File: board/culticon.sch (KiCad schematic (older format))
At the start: 32 parts

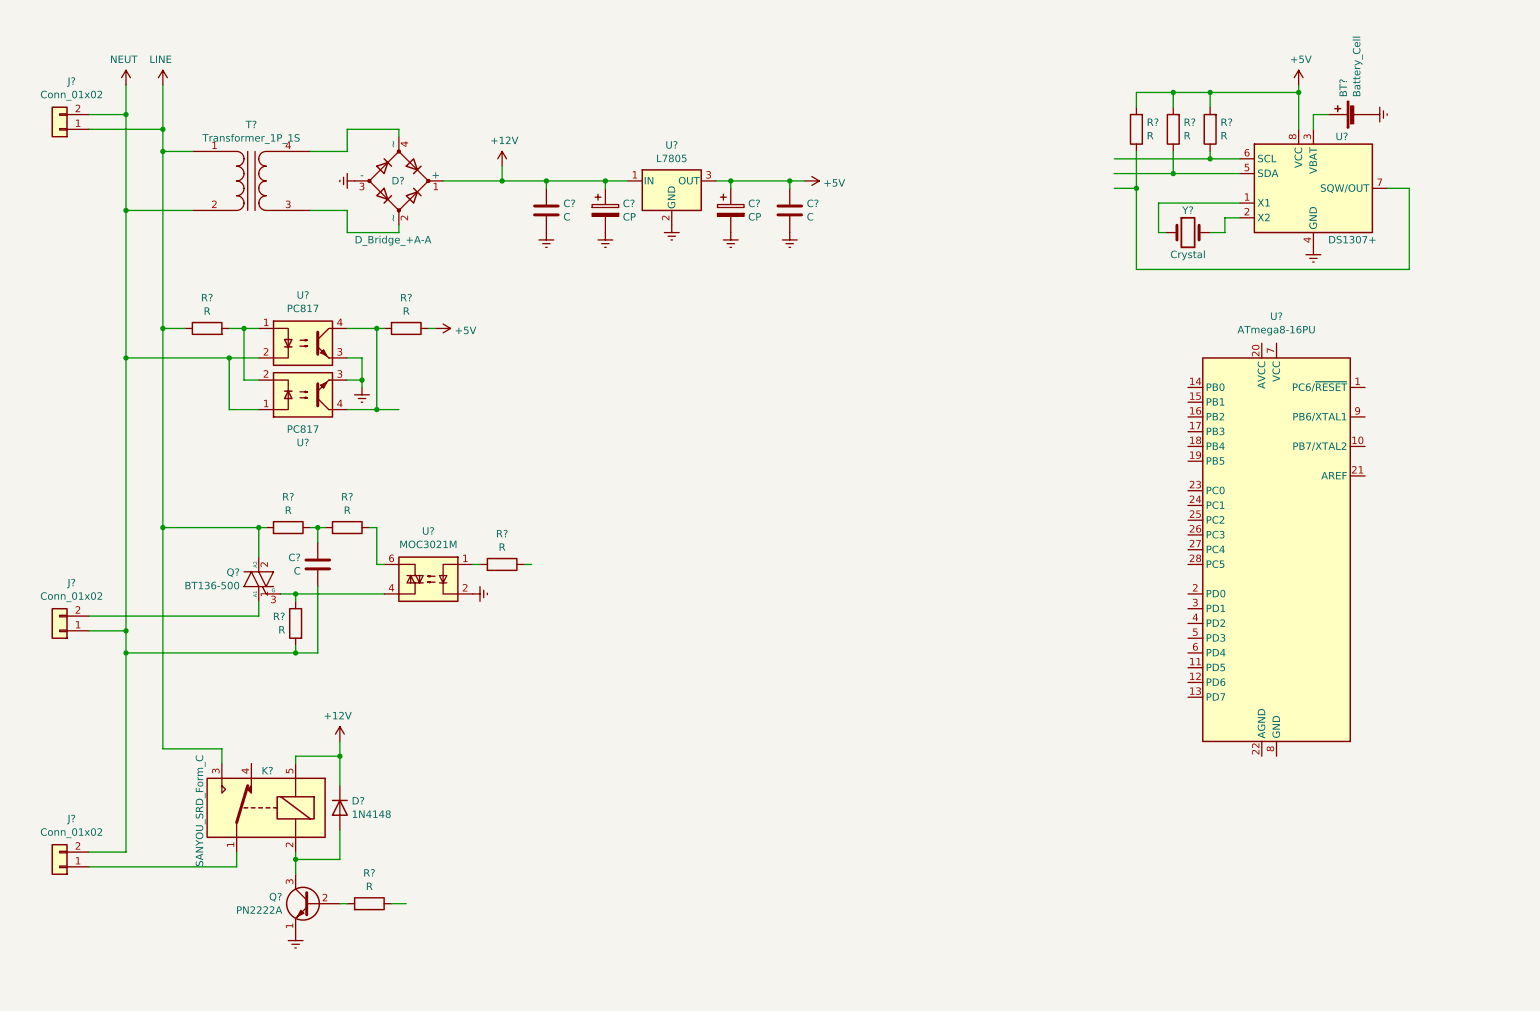
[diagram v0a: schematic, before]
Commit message: minimal working schem
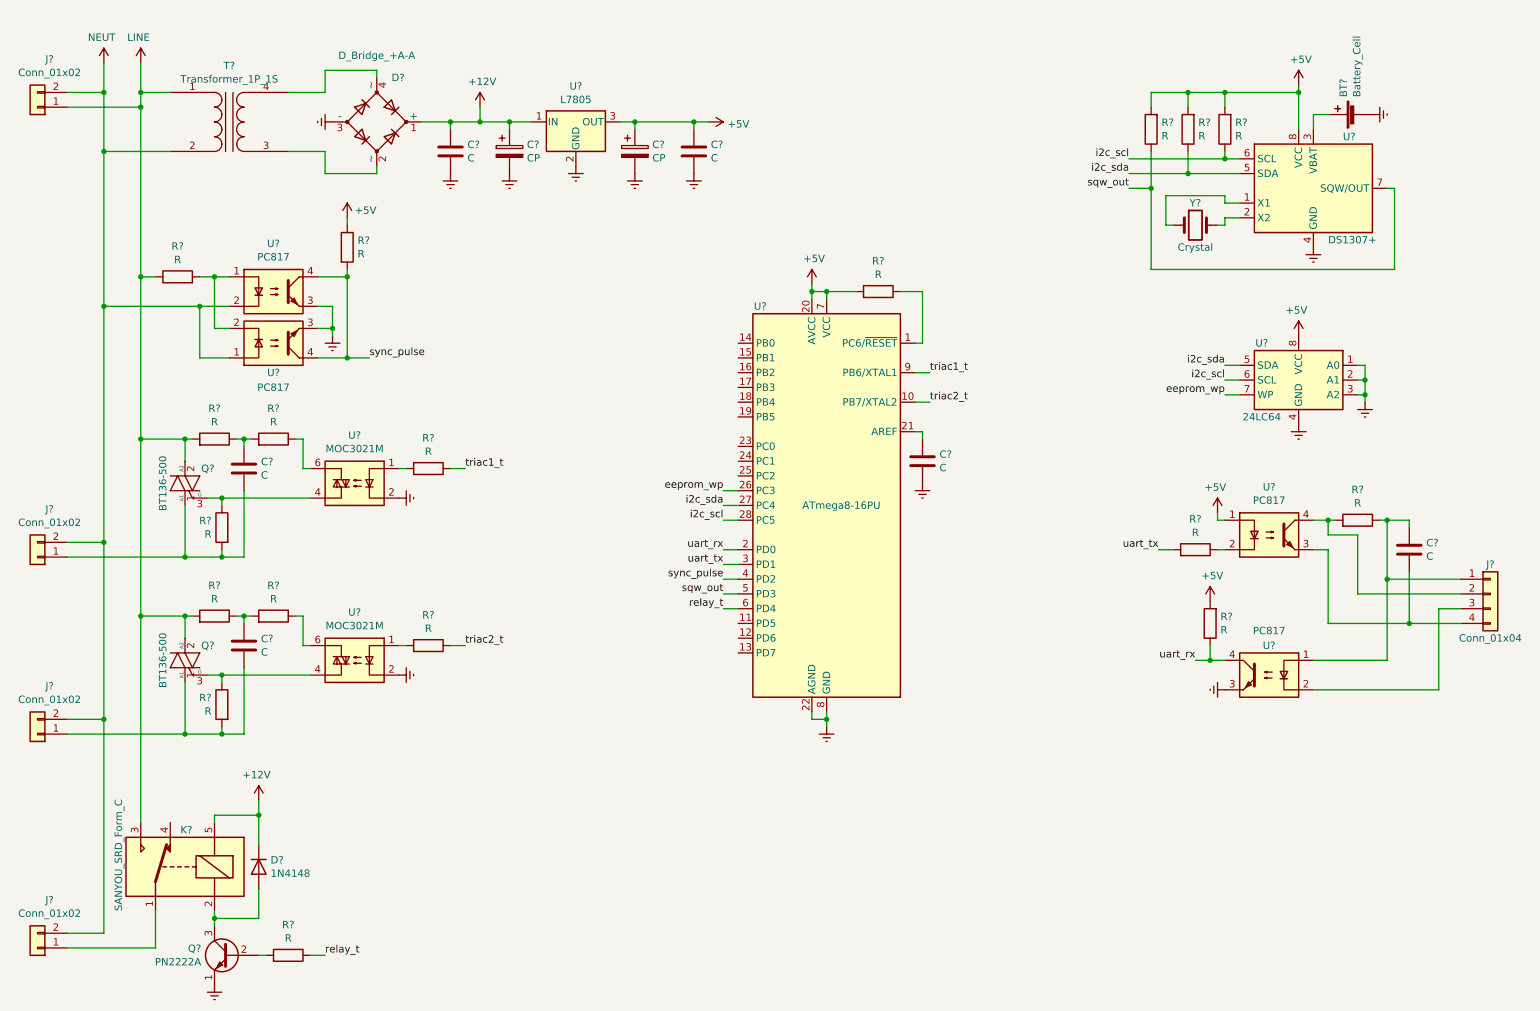
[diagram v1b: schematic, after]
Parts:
- removed R?: R, symbol Device:R
- added C? (x3): C, symbol Device:C
- added J?: Conn_01x02, symbol Connector_Generic:Conn_01x02
- added J?: Conn_01x04, symbol Connector_Generic:Conn_01x04
- added Q?: BT136-500, Package_TO_SOT_THT:TO-220-3_Vertical, symbol Triac_Thyristor:BT136-500
- added R? (x9): R, symbol Device:R
- added U?: MOC3021M, symbol Relay_SolidState:MOC3021M
- added U?: 24LC64, symbol Memory_EEPROM:24LC64
- added U? (x2): PC817, Package_DIP:DIP-4_W7.62mm, symbol Isolator:PC817
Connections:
- net labels added: eeprom_wp, i2c_scl, i2c_sda, relay_t, sqw_out, sync_pulse, triac1_t, triac2_t, uart_rx, uart_tx
- wire segments 118 -> 201
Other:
- moved on the sheet: C?, D?, J?, K?, Q?, R?, T?, U?, Y?

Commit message: complete dev schem
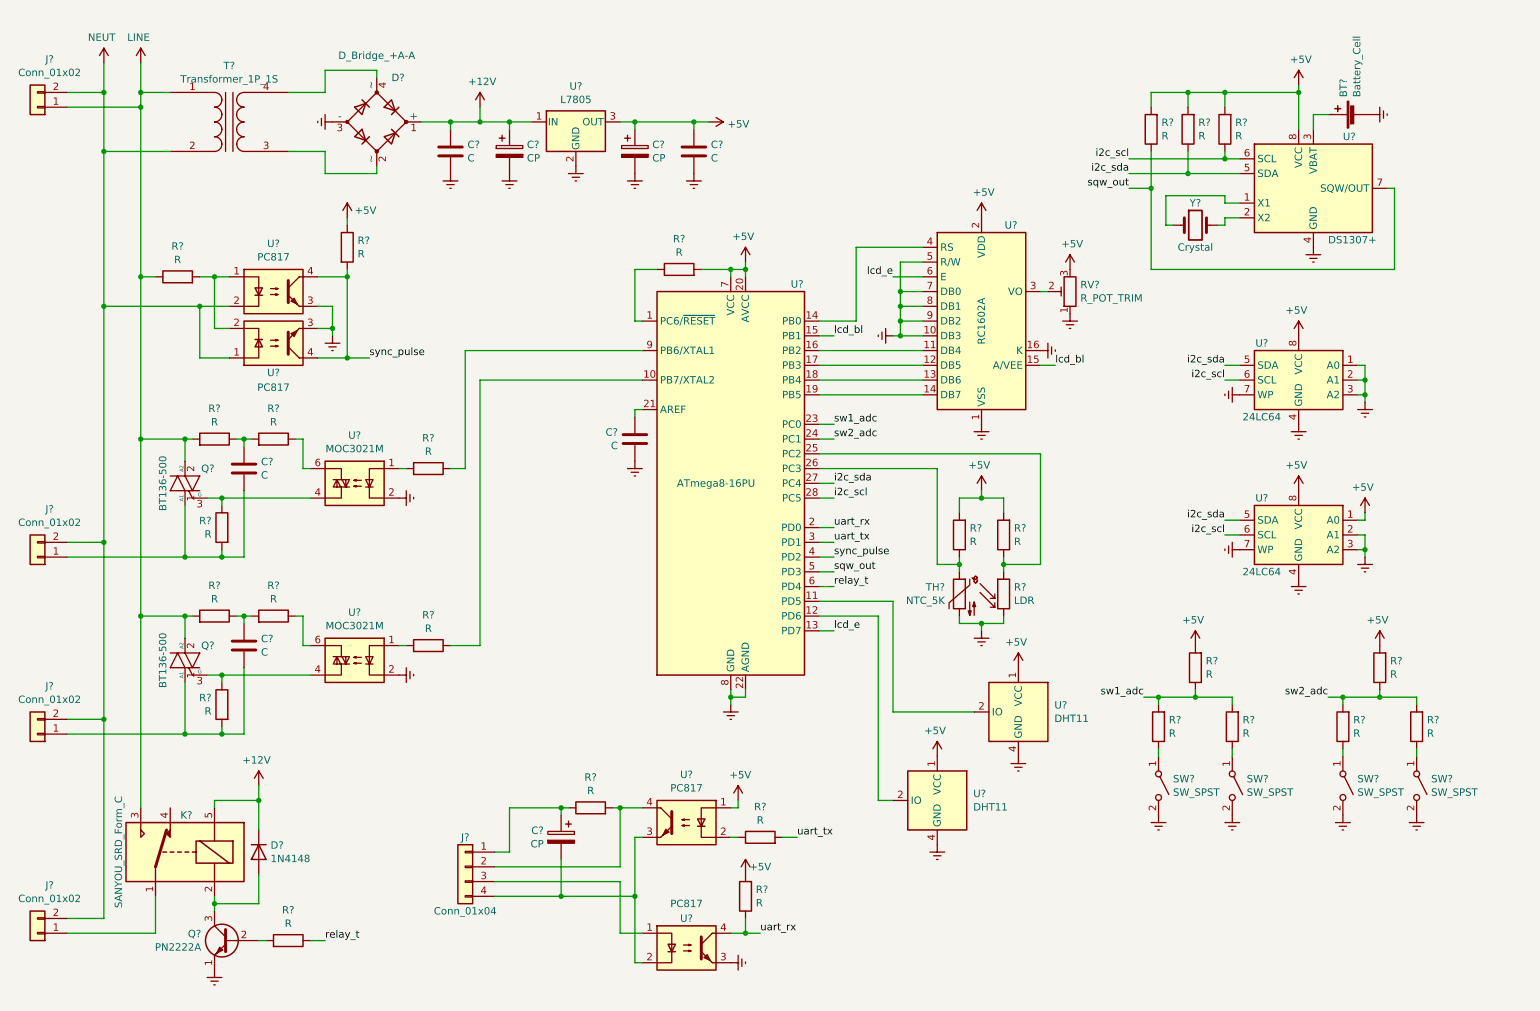
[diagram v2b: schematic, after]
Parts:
- removed C?: C, symbol Device:C
- removed R?: R, symbol Device:R
- added C?: CP, symbol Device:CP
- added R? (x9): R, symbol Device:R
- added R?: LDR, symbol Device:R_PHOTO
- added RV?: R_POT_TRIM, symbol Device:R_POT_TRIM
- added SW? (x4): SW_SPST, symbol Switch:SW_SPST
- added TH?: NTC_5K, symbol Device:Thermistor_NTC
- added U?: RC1602A, Display:RC1602A, symbol Display_Character:RC1602A
- added U?: 24LC64, symbol Memory_EEPROM:24LC64
- added U? (x2): DHT11, Sensor:Aosong_DHT11_5.5x12.0_P2.54mm, symbol Sensor:DHT11
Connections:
- net +5V: now also R?.2, R?.2, R?.2, R?.2, RV?.3, U?.1 (A0), U?.1 (VCC), U?.1 (VCC), U?.2 (VDD), U?.8 (VCC)
- net Earth: now also U?.7 (WP), R?.2, RV?.1, SW?.2 (B), SW?.2 (B), SW?.2 (B), SW?.2 (B), TH?.2, U?.1 (VSS), U?.10 (DB3), U?.16 (K), U?.2 (A1), U?.3 (A2), U?.4 (GND), U?.4 (GND), U?.4 (GND), U?.5 (R/W), U?.7 (DB0), U?.7 (WP), U?.8 (DB1), U?.9 (DB2)
- net i2c_scl: now also U?.6 (SCL)
- net i2c_sda: now also U?.5 (SDA)
- net at U?.11 (PD5): now also U?.2 (IO)
- net at U?.12 (PD6): now also U?.2 (IO)
- net lcd_e: now reaches U?.13 (PD7)
- net lcd_e: now also U?.6 (E)
- net at U?.14 (PB0): now also U?.4 (RS)
- net lcd_bl: now reaches U?.15 (PB1)
- net lcd_bl: now also U?.15 (A/VEE)
- net at U?.16 (PB2): now also U?.11 (DB4)
- net at U?.17 (PB3): now also U?.12 (DB5)
- net at U?.18 (PB4): now also U?.13 (DB6)
- net at U?.19 (PB5): now also U?.14 (DB7)
- net sw1_adc: now reaches U?.23 (PC0)
- net sw1_adc: now also R?.1, R?.2, R?.2
- net sw2_adc: now reaches U?.24 (PC1)
- net sw2_adc: now also R?.1, R?.2, R?.2
- net at U?.25 (PC2): now also R?.1, R?.1
- net at J?.4 (Pin_4), U?.3: now also U?.2, C?.2
- net at J?.2 (Pin_2), U?.4: now also R?.2
- net at U?.1: now also J?.3 (Pin_3); no longer J?.1 (Pin_1)
- net eeprom_wp: no longer names the net of U?.26 (PC3)
- net eeprom_wp: now also R?.1, TH?.1; no longer U?.7 (WP)
- net triac1_t: no longer names the net of R?.1, U?.9 (PB6/XTAL1)
- net triac2_t: no longer names the net of R?.1, U?.10 (PB7/XTAL2)
- new net: C?.1, J?.1 (Pin_1), R?.1
- new net: RV?.2, U?.3 (VO)
- new net: R?.1, SW?.1 (A) (x4)
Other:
- moved on the sheet: C?, D?, J?, K?, Q?, R?, U?
